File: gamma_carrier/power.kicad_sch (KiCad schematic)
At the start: 8 parts

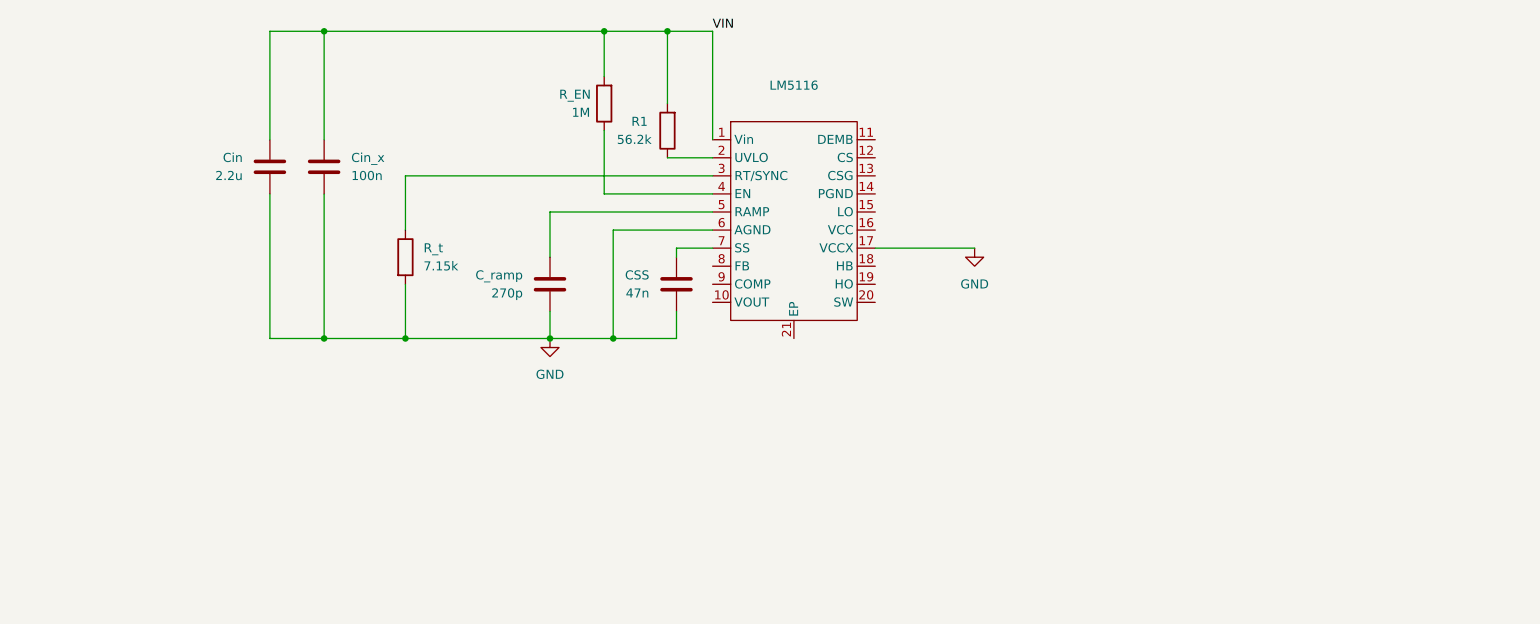
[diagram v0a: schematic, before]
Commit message: lm5116 done, not checked yet
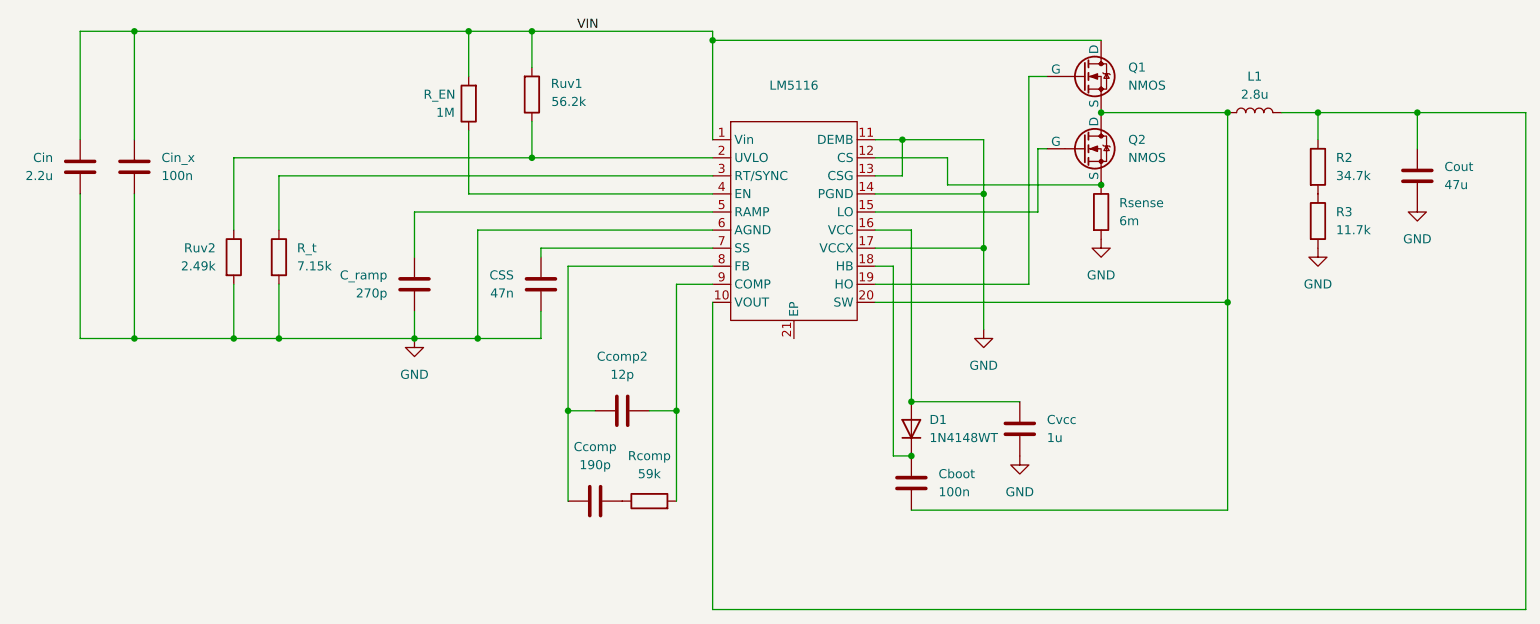
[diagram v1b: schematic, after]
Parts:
- added Cboot: 100n, symbol Device:C
- added Ccomp: 190p, symbol Device:C
- added Ccomp2: 12p, symbol Device:C
- added Cout: 47u, symbol Device:C
- added Cvcc: 1u, symbol Device:C
- added D1: 1N4148WT, Diode_SMD:D_SOD-523, symbol Diode:1N4148WT
- added L1: 2.8u, symbol Device:L
- added Q1, Q2: NMOS, symbol Simulation_SPICE:NMOS
- added R2: 34.7k, symbol Device:R
- added R3: 11.7k, symbol Device:R
- added Rcomp: 59k, symbol Device:R
- added Rsense: 6m, symbol Device:R
- added Ruv2: 2.49k, symbol Device:R
- renumbered R1 to Ruv1
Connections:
- net GND: now also LM5116.11 (DEMB), LM5116.13 (CSG), LM5116.14 (PGND), Cout.2, Cvcc.2, R3.2, Rsense.2, Ruv2.2
- net VIN: now also Q1.1 (D)
- net at LM5116.10 (VOUT): now also Cout.1, L1.2, R2.1
- net at LM5116.12 (CS): now also Q2.3 (S), Rsense.1
- net at LM5116.15 (LO): now also Q2.2 (G)
- net at LM5116.16 (VCC): now also Cvcc.1, D1.2 (A)
- net at LM5116.18 (HB): now also Cboot.1, D1.1 (K)
- net at LM5116.19 (HO): now also Q1.2 (G)
- net at LM5116.2 (UVLO), Ruv1.1: now also Ruv2.1
- net at LM5116.20 (SW): now also Cboot.2, L1.1, Q1.3 (S), Q2.1 (D)
- net at LM5116.8 (FB): now also Ccomp.2, Ccomp2.1
- net at LM5116.9 (COMP): now also Ccomp2.2, Rcomp.2
- new net: Ccomp.1, Rcomp.1
- new net: R2.2, R3.1
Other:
- moved on the sheet: CSS, C_ramp, Cin, Cin_x, R_EN, R_t, Ruv1
